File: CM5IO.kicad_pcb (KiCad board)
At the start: 4 copper layers, 58 parts, among them J1 USB3_A, J11 USB_C_Receptacle_USB2.0, J14 JST_SHBM04B-SRSS-TB, J2 Conn_02x07_Odd_Even, J22 690-019-298-412, J3 Conn_01x03, J4 Bus_M.2_Socket_M, J8 THD-20-R, SW1 Right angle Tact button, U12 RT9742SNGV, U5 74LVC1G07SE-7, U6 AP22653W6, U7 ASEK-32.768KHZ-L-R-T, U8 AP3441SHE-7B

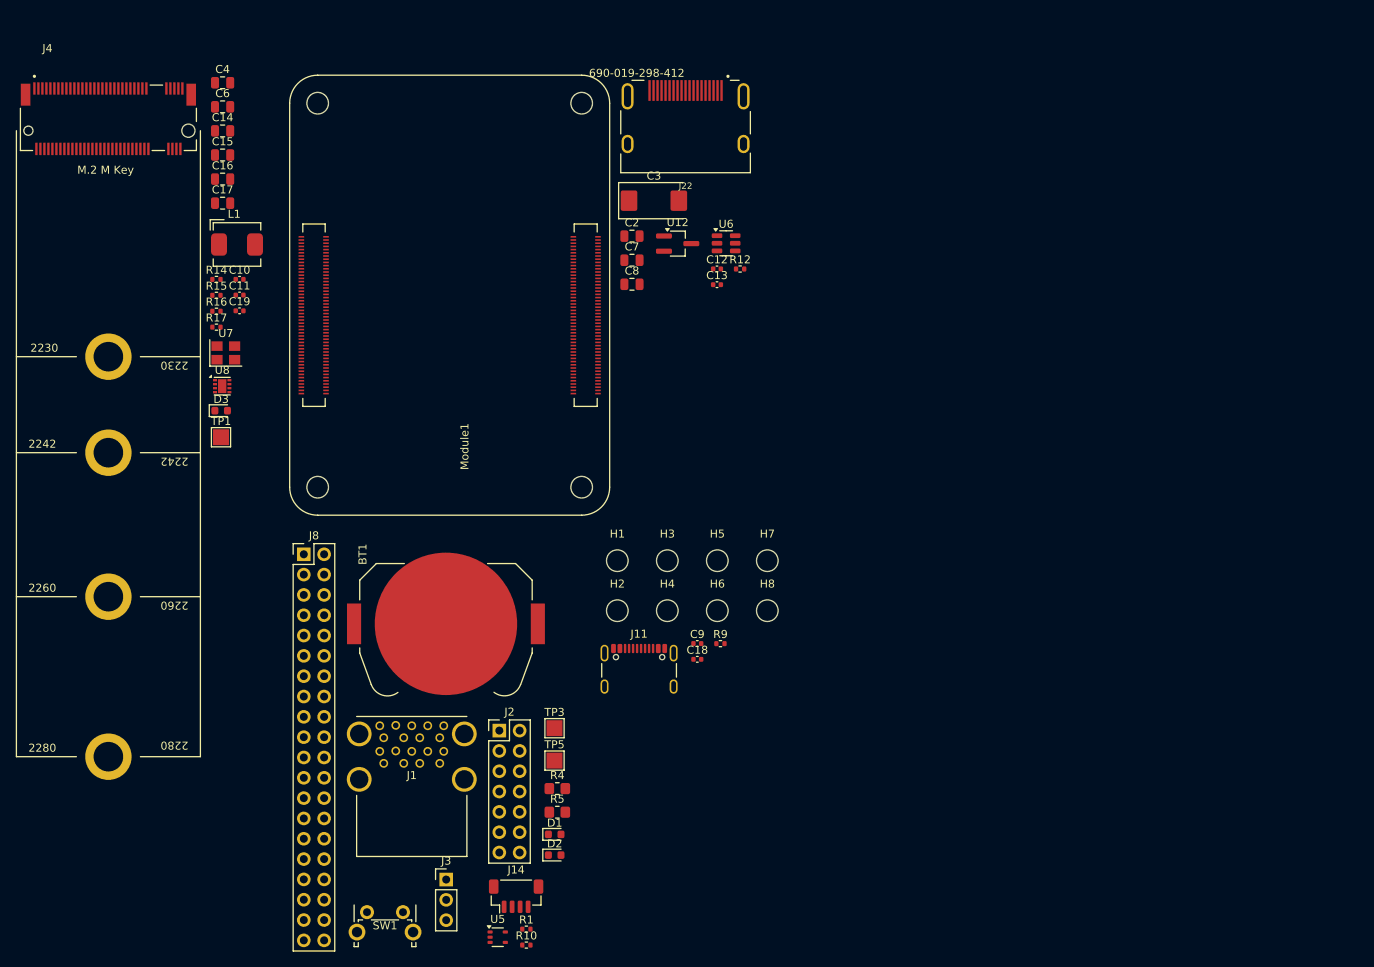
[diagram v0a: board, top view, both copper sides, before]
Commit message: Board development
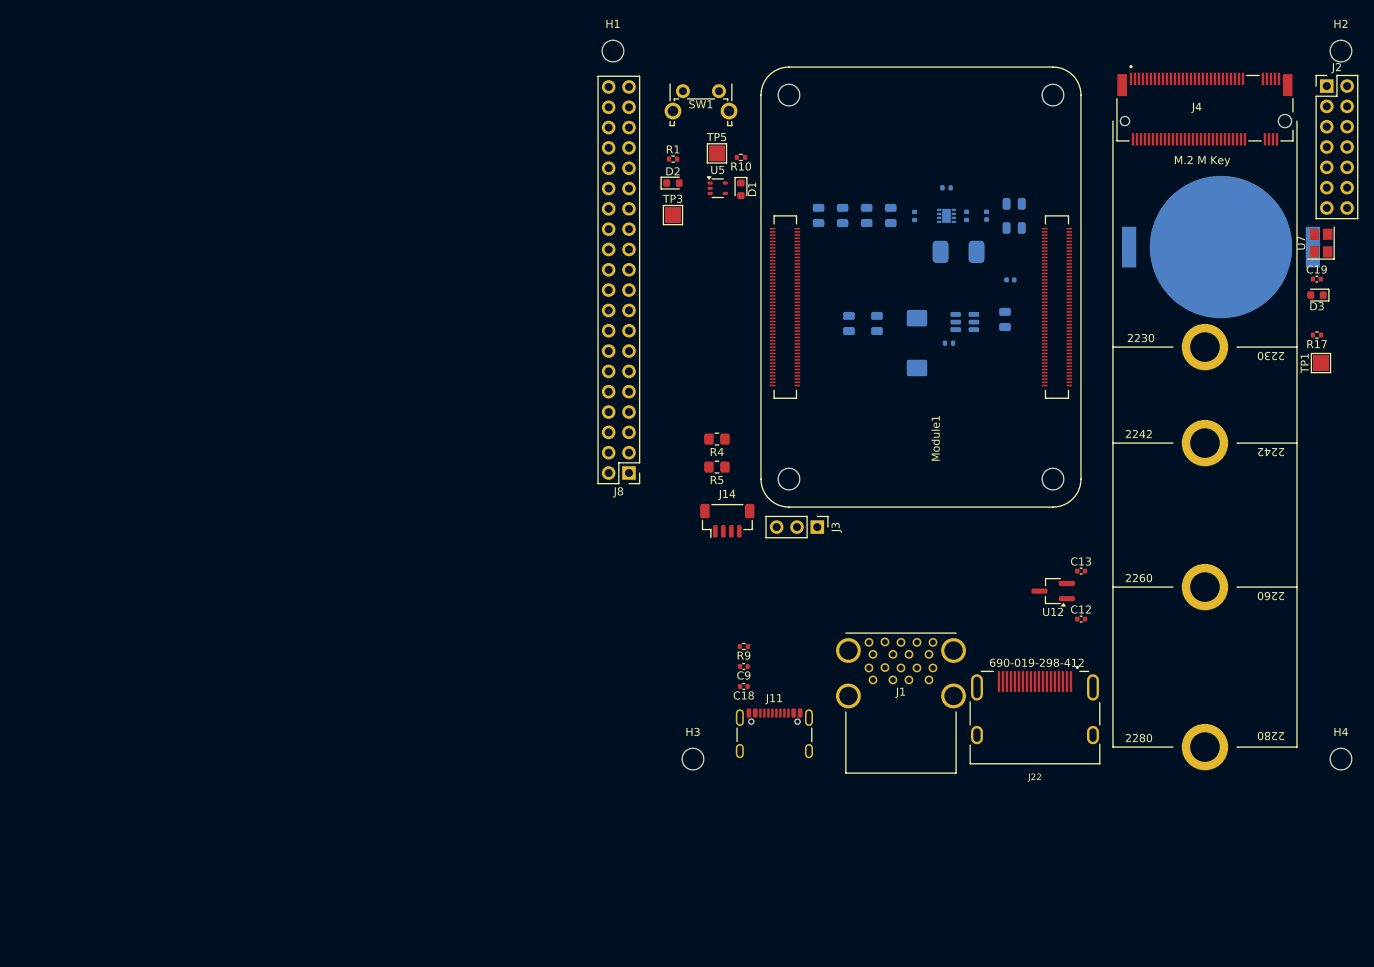
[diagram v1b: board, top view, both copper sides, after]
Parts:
- removed H5, H6, H7, H8: MountingHole, CM5IO:MountingHole_2.7mm_M2.5_DIN965
- BT1, C10, C11, C14, C15, C16, C17, C2, C3, C4, C6, C7, C8, L1, R12, R14, R15, R16, U6, U8: moved to B.Cu
- moved TP1 137.8 mm to (215.0, 82.7), turned to 90 degrees
- moved D3 137.7 mm to (214.5, 74.2), turned to 180 degrees
- moved U7 137.6 mm to (215.0, 67.7), turned to 90 degrees
- moved R17 137.6 mm to (214.5, 79.2), turned to 180 degrees
- moved J4 137.1 mm to (200.5, 52.5)
- moved C19 134.7 mm to (214.5, 72.2)
- moved J2 131.1 mm to (215.7, 48.1)
- moved H2 114.3 mm to (217.5, 43.7)
- moved SW1 110.0 mm to (135.2, 48.7)
- moved BT1 107.7 mm to (202.5, 68.2), turned to 180 degrees
- moved R10 102.1 mm to (142.5, 57.0), turned to 180 degrees
- moved C4 100.1 mm to (176.6, 62.8), turned to 180 degrees
- moved C6 100.1 mm to (176.6, 65.8), turned to 180 degrees
- moved R1 98.0 mm to (134.0, 57.2)
- moved U5 97.6 mm to (139.6, 60.8)
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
